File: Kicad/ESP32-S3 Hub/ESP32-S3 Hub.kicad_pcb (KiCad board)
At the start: 6 copper layers, 15 x 30 mm, 61 parts, among them J1 1.27mm 3pin socket, J10 1.27mm 3pin socket, J11 7 pin FPC 0.3mm Panasonic Y3b, J12 1.27mm 3pin socket, J13 TE 3-2363961-0 receptacle, J14 TE 3-2363962-0 Connector, J16 TE 3-2363961-0 receptacle, J17 TE 3-2363962-0 Connector, J2 1.27mm 3pin socket, J21 1.27mm 4 pin socket, J22 1.27mm 4 pin header, J3 7 pin FPC 0.3mm Panasonic Y3b, J4 1.27mm 3pin socket, J5 7 pin FPC 0.3mm Panasonic Y3b, J6 1.27mm 3pin socket, J7 1.27mm 3pin socket, J8 7 pin FPC 0.3mm Panasonic Y3b, J9 1.27mm 3pin socket, SW1 Mitsumi R-667996, SW2 Mitsumi R-667996, U1 ESP32-S3, U2 74HC595, U3 THVD1420DRLR, Y1 ABM11-40.000MHZ-B1U-T3, 10ppm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

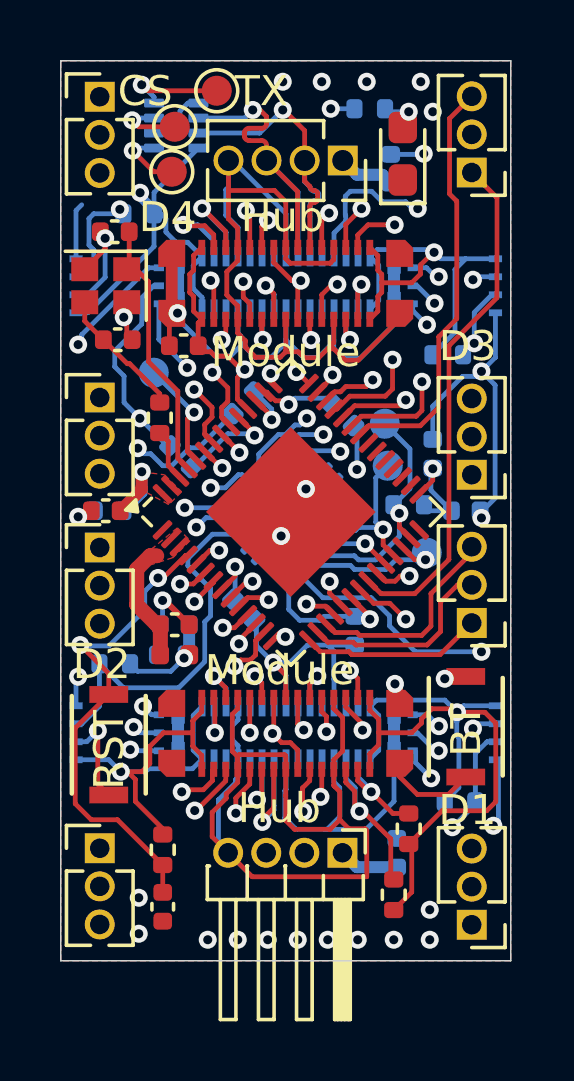
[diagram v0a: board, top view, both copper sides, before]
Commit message: Tweaked some tracks
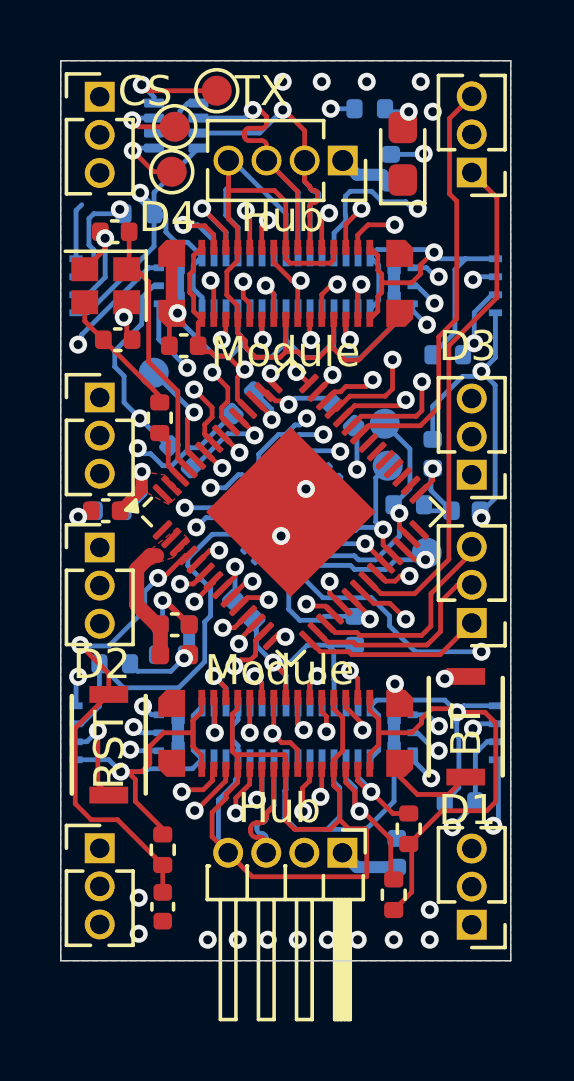
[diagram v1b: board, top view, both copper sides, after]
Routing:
- net RS485-: track 62.5 -> 64.4 mm, vias 4 -> 3
